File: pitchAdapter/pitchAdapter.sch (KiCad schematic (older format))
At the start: 4 parts, among them J1 CONN_02X09, J2 CONN_02X09, J3 CONN_02X09, J4 CONN_02X09

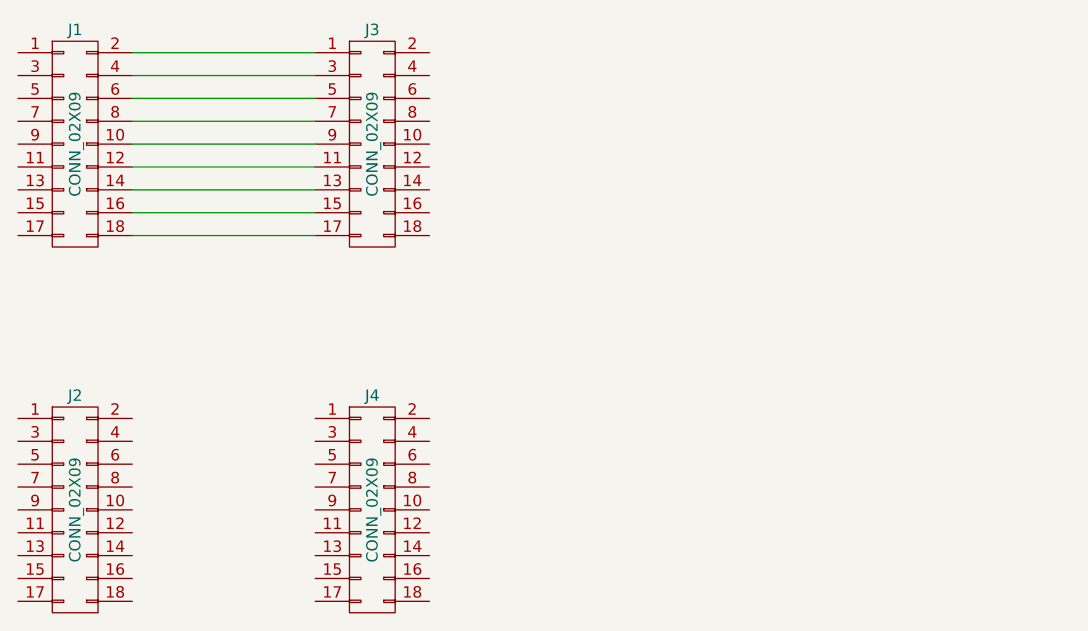
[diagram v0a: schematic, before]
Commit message: Adpter V1 Done
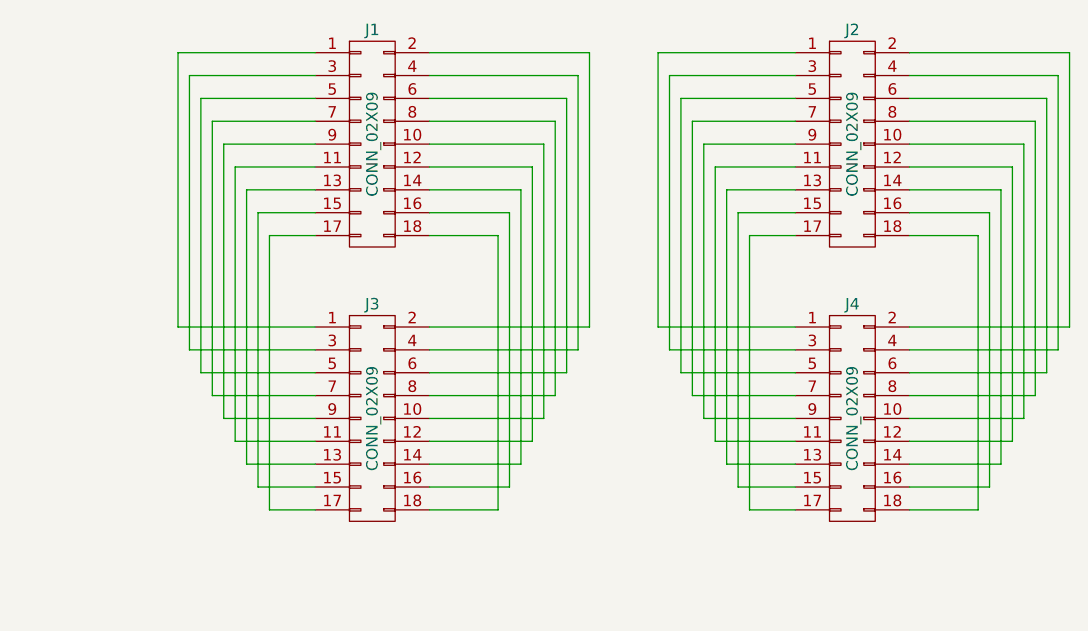
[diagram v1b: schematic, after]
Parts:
- J1: renamed from J3; footprint (none) -> Socket_Strips:Socket_Strip_Straight_2x09_Pitch2.00mm
- J2: footprint (none) -> Pin_Headers:Pin_Header_Straight_2x09_Pitch2.00mm
- J3: renamed from J1; footprint (none) -> Socket_Strips:Socket_Strip_Straight_2x09_Pitch2.54mm
- J4: footprint (none) -> Pin_Headers:Pin_Header_Straight_2x09_Pitch2.54mm
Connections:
- net at J3.1 (P1): now also J1.1 (P1)
- net at J3.10 (P10): now also J1.10 (P10); no longer J1.9 (P9)
- net at J3.11 (P11): now also J1.11 (P11)
- net at J3.12 (P12): now also J1.12 (P12); no longer J1.11 (P11)
- net at J3.13 (P13): now also J1.13 (P13)
- net at J3.14 (P14): now also J1.14 (P14); no longer J1.13 (P13)
- net at J3.15 (P15): now also J1.15 (P15)
- net at J3.16 (P16): now also J1.16 (P16); no longer J1.15 (P15)
- net at J3.17 (P17): now also J1.17 (P17)
- net at J3.18 (P18): now also J1.18 (P18); no longer J1.17 (P17)
- net at J3.2 (P2): now also J1.2 (P2); no longer J1.1 (P1)
- net at J3.3 (P3): now also J1.3 (P3)
- net at J3.4 (P4): now also J1.4 (P4); no longer J1.3 (P3)
- net at J3.5 (P5): now also J1.5 (P5)
- net at J3.6 (P6): now also J1.6 (P6); no longer J1.5 (P5)
- net at J3.7 (P7): now also J1.7 (P7)
- net at J3.8 (P8): now also J1.8 (P8); no longer J1.7 (P7)
- net at J3.9 (P9): now also J1.9 (P9)
- net at J2.1 (P1): now also J4.1 (P1)
- net at J2.10 (P10): now also J4.10 (P10)
- net at J2.11 (P11): now also J4.11 (P11)
- net at J2.12 (P12): now also J4.12 (P12)
- net at J2.13 (P13): now also J4.13 (P13)
- net at J2.14 (P14): now also J4.14 (P14)
- net at J2.15 (P15): now also J4.15 (P15)
- net at J2.16 (P16): now also J4.16 (P16)
- net at J2.17 (P17): now also J4.17 (P17)
- net at J2.18 (P18): now also J4.18 (P18)
- net at J2.2 (P2): now also J4.2 (P2)
- net at J2.3 (P3): now also J4.3 (P3)
- net at J2.4 (P4): now also J4.4 (P4)
- net at J2.5 (P5): now also J4.5 (P5)
- net at J2.6 (P6): now also J4.6 (P6)
- net at J2.7 (P7): now also J4.7 (P7)
- net at J2.8 (P8): now also J4.8 (P8)
- net at J2.9 (P9): now also J4.9 (P9)
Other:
- moved on the sheet: J3
